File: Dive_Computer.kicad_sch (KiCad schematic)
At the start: 30 parts, among them IC1 LTC4120EUD-4.2#PBF, IC2 MS583730BA01-50, J1 SCREEN, U1 ESP32-C3_SUPERMINI_TH

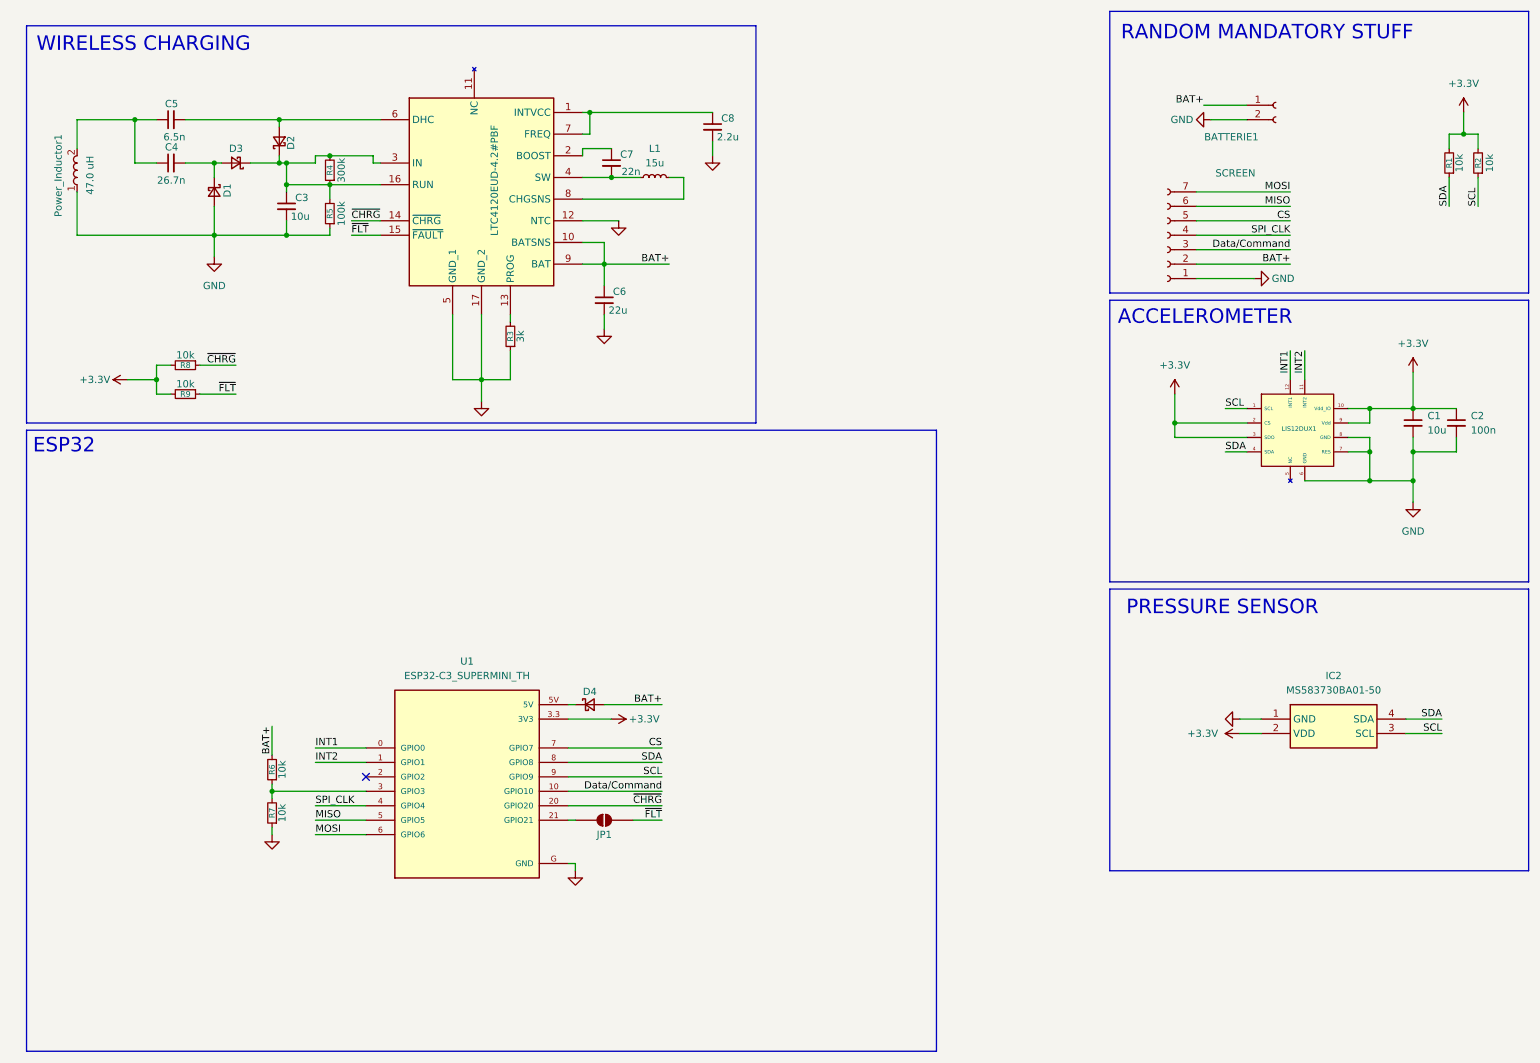
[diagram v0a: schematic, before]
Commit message: Schematic update
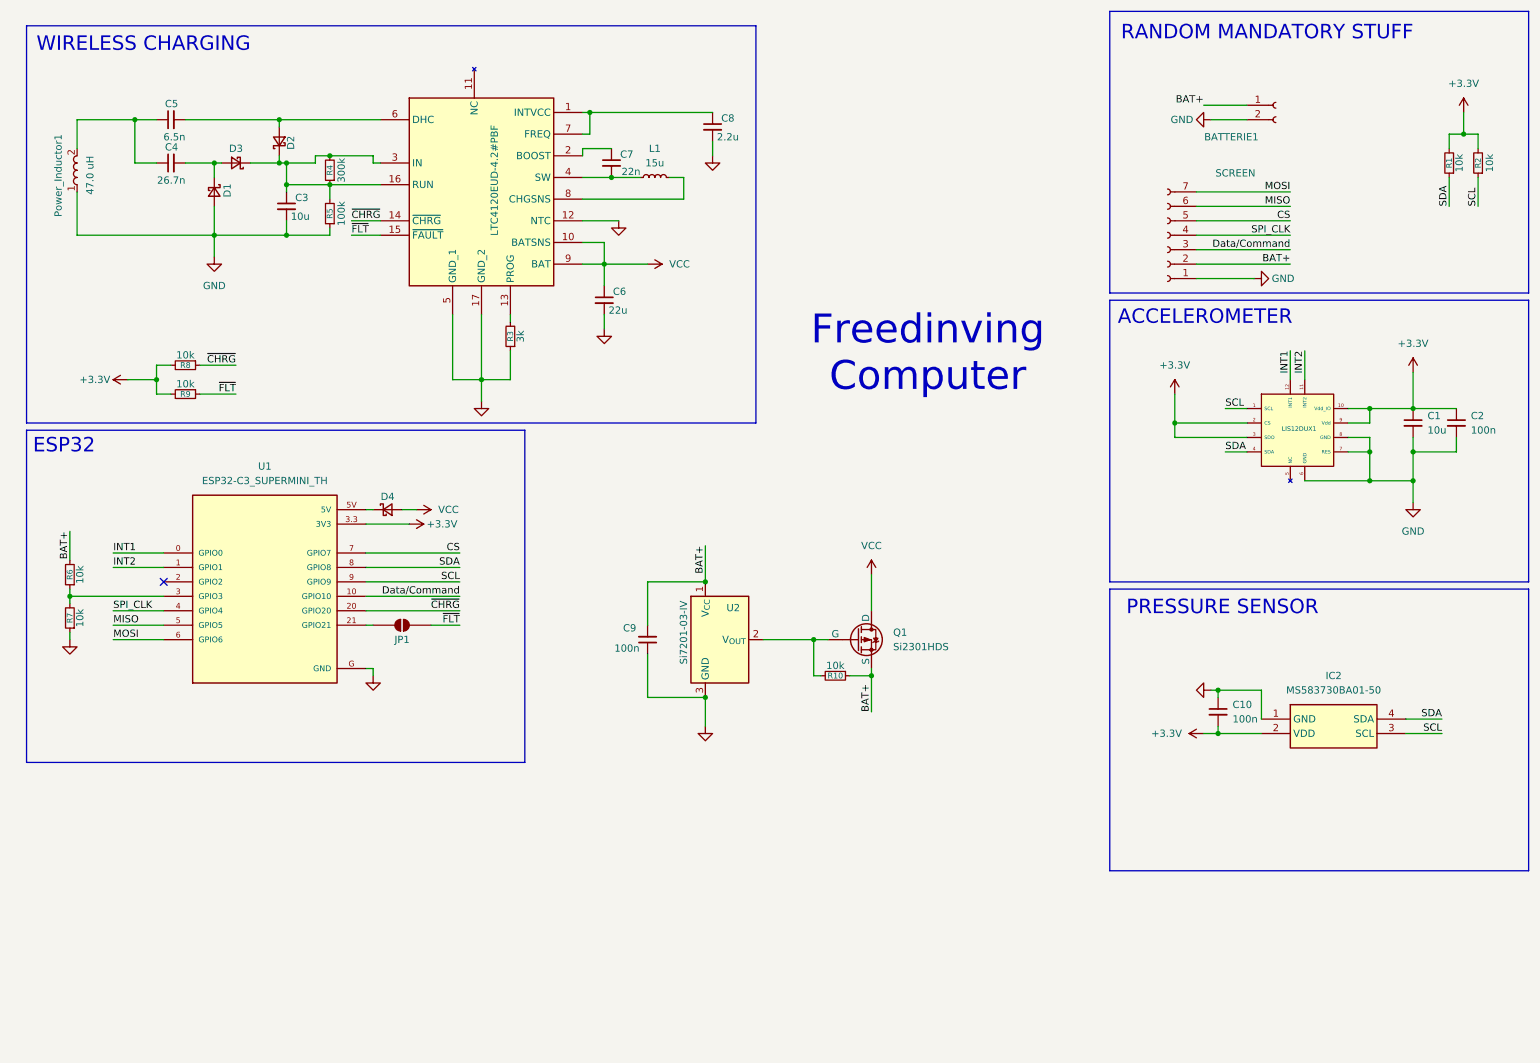
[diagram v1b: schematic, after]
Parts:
- added C10, C9: 100n, Capacitor_SMD:C_0603_1608Metric, symbol Device:C_Small
- added Q1: Si2301HDS, Package_TO_SOT_SMD:TSOT-23, symbol Simulation_SPICE:PMOS
- added R10: 10k, Resistor_SMD:R_0603_1608Metric, symbol Device:R_Small
- added U2: Si7201-03-IV, Package_TO_SOT_SMD:SOT-23, symbol Sensor_Magnetic:A1102xLH
- C1, C3, C6: footprint (none) -> Capacitor_SMD:C_1210_3225Metric
- C2, C4, C5, C7, C8: footprint (none) -> Capacitor_SMD:C_0603_1608Metric
- D1, D2, D3, D4: footprint (none) -> Diode_SMD:D_MicroSMP_LargeCathode
- JP1: footprint (none) -> Jumper:SolderJumper-2_P1.3mm_Open_RoundedPad1.0x1.5mm
- L1: footprint (none) -> Inductor_SMD:L_APV_ANR4018
- Power_Inductor1: footprint Inductor_THT_Wurth:L_Wurth_WE-WPCC-RX_760308101303 -> Connector_PinHeader_2.54mm:PinHeader_1x02_P2.54mm_Vertical
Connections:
- net +3.3V: now also C10.2
- net BAT+: now also C9.2, Q1.3 (S), R10.1, U2.1 (V_{CC}); no longer C6.1, D4.2 (A), IC1.10 (BATSNS), IC1.9 (BAT)
- net GND: now also C10.1, C9.1, U2.3 (GND)
- new net: Q1.2 (G), R10.2, U2.2 (V_{OUT})
- new net VCC: C6.1, D4.2 (A), IC1.10 (BATSNS), IC1.9 (BAT), Q1.1 (D)
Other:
- note added: "Freedinving Computer"
- moved on the sheet: D4, JP1, R6, R7, U1
